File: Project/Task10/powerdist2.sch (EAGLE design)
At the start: 51 parts

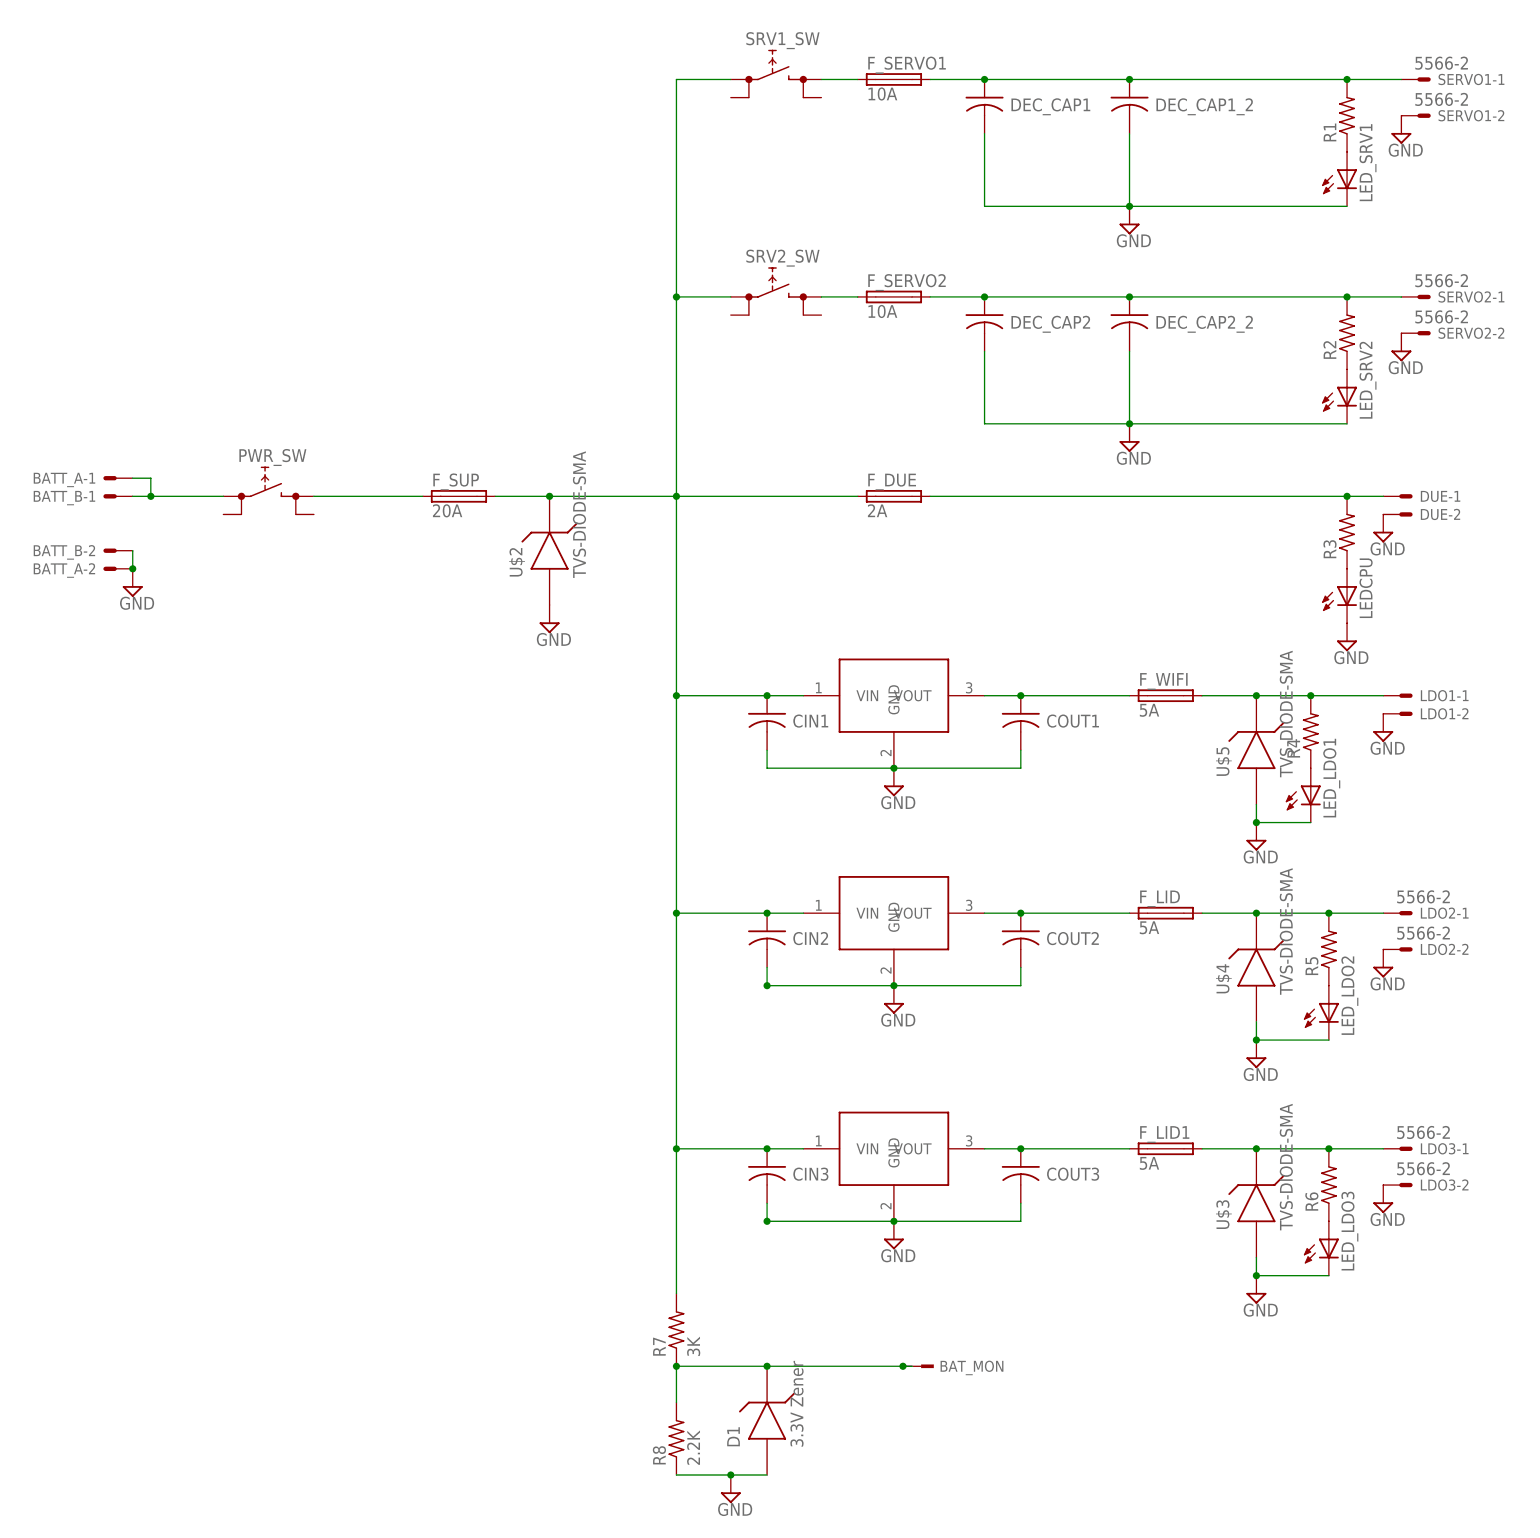
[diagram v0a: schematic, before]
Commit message: Updated Schematic, ready for submitting...
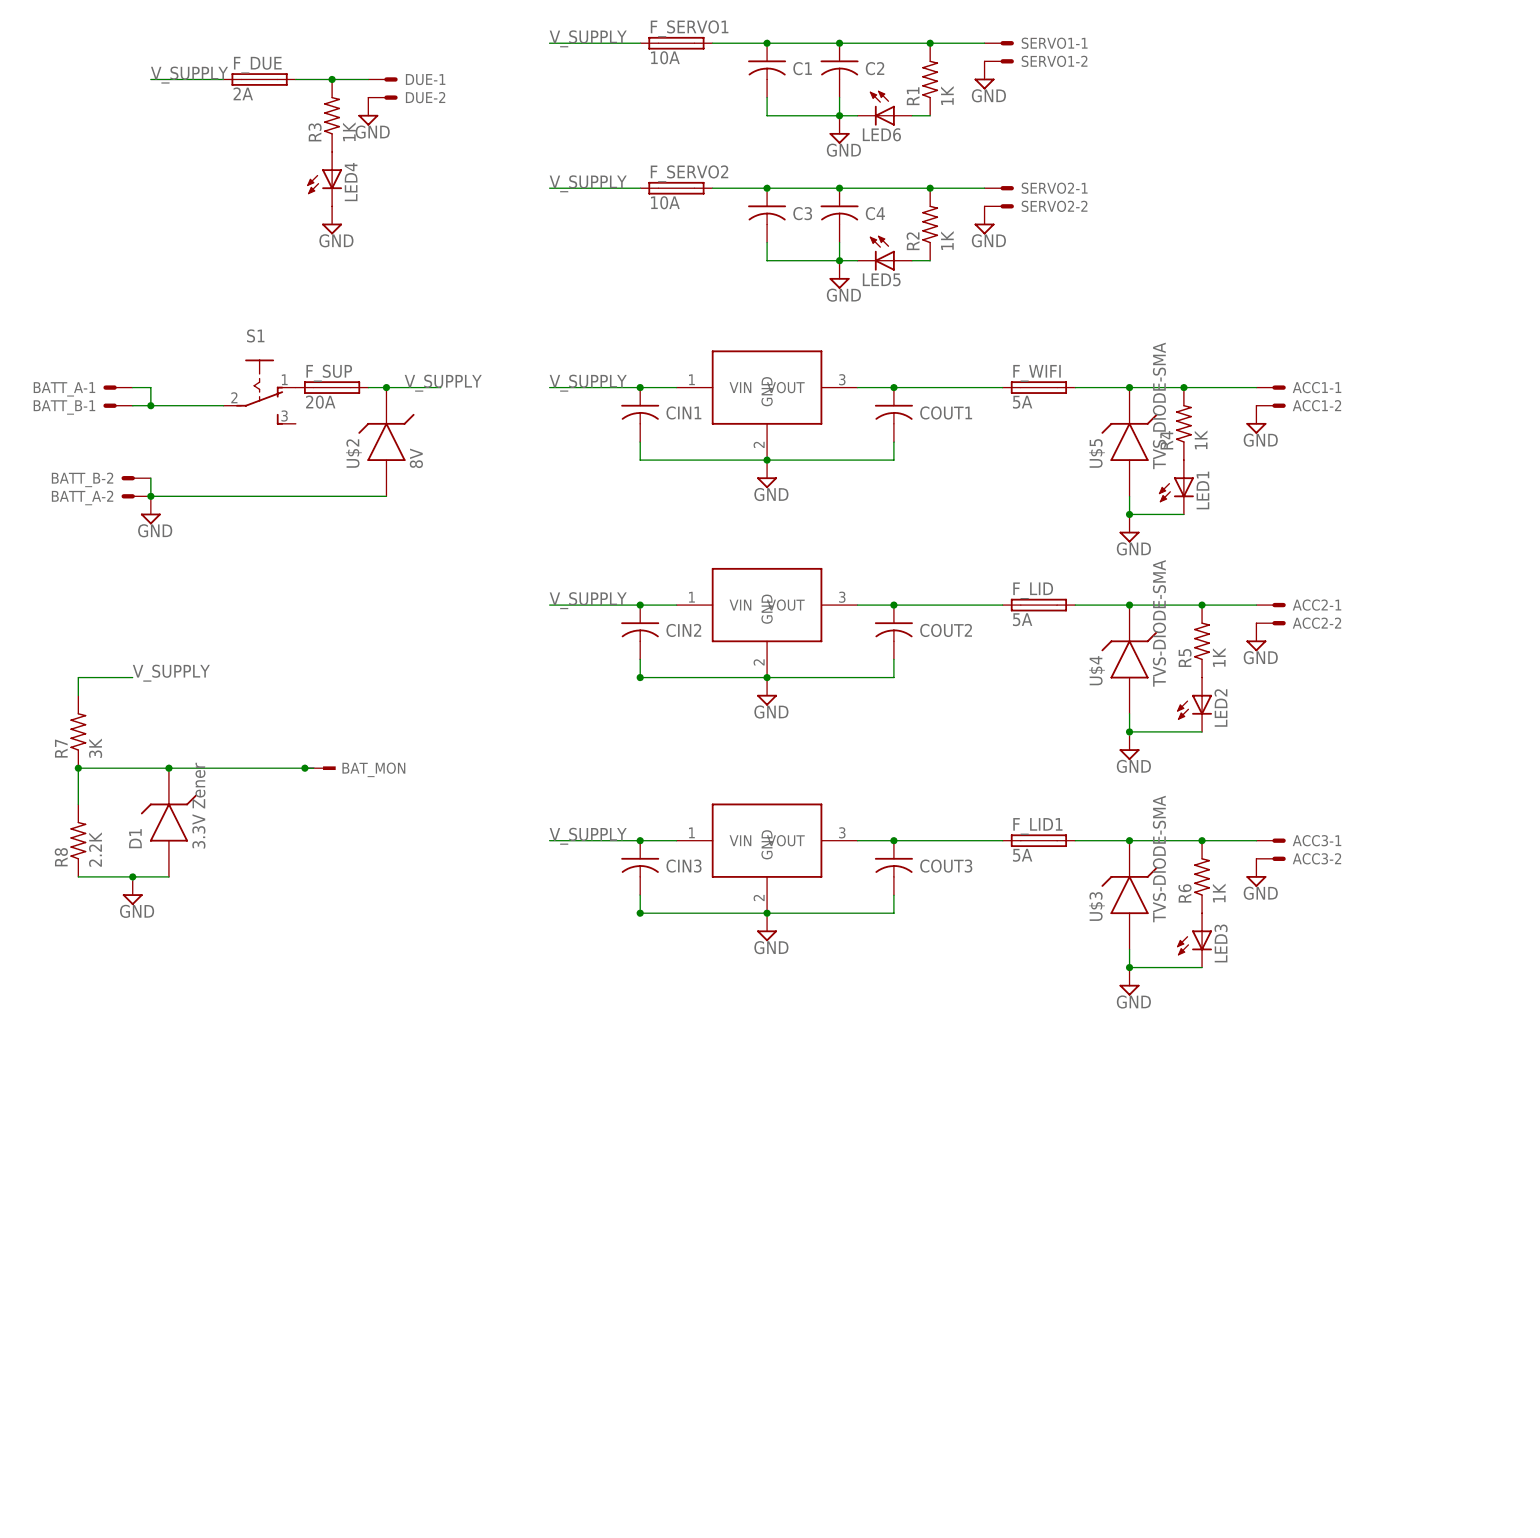
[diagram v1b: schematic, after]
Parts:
- removed DEC_CAP1, DEC_CAP1_2, DEC_CAP2, DEC_CAP2_2: CAPACITORTH_CAP, TinyGadget(1):CAPACITORTH_CAP
- removed LDO1: C-GRID-02-70553, con-molex:C-GRID-02-70553
- removed LDO2, LDO3: 5566-2, con-molex:5566-2
- removed LEDCPU, LED_LDO1, LED_LDO2, LED_LDO3, LED_SRV1, LED_SRV2: (no value), led:LEDCHIP-LED0805
- removed PWR_SW, SRV1_SW, SRV2_SW: (no value), switch:REKN
- added ACC1: C-GRID-02-70553, con-molex:C-GRID-02-70553
- added ACC2, ACC3: 5566-2, con-molex:5566-2
- added C1, C2, C3, C4: CAPACITORTH_CAP, TinyGadget(1):CAPACITORTH_CAP
- added LED1, LED2, LED3, LED4, LED5, LED6: (no value), led:LEDCHIP-LED0805
- added S1: (no value), switch:255SB
- R1, R2, R3, R4, R5, R6: value (none) -> 1K
- U$2: value TVS-DIODE-SMA -> 8V
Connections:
- removed net N$17: F_SERVO2.1, SRV2_SW.1@A
- removed net N$20: CIN1.1, CIN2.1, CIN3.1, F_DUE.1, F_SUP.2, R7.2, SRV1_SW.0@A, SRV2_SW.0@A, U$1.VIN, U$2.CAT, U$6.VIN, U$7.VIN
- removed net N$3: F_SERVO1.1, SRV1_SW.1@A
- new net V_SUPPLY: CIN1.1, CIN2.1, CIN3.1, F_DUE.1, F_SERVO1.1, F_SERVO2.1, F_SUP.2, R7.2, U$1.VIN, U$2.CAT, U$6.VIN, U$7.VIN
- net GND: now also ACC1-2.S, ACC2-2.S, ACC3-2.S, C1.2, C2.2, C3.2, C4.2, LED1.C, LED2.C, LED3.C, LED4.C, LED5.C, LED6.C; no longer DEC_CAP1.2, DEC_CAP1_2.2, DEC_CAP2.2, DEC_CAP2_2.2, LDO1-2.S, LDO2-2.S, LDO3-2.S, LEDCPU.C, LED_LDO1.C, LED_LDO2.C, LED_LDO3.C, LED_SRV1.C, LED_SRV2.C
- net N$1: now also C3.1, C4.1; no longer DEC_CAP2.1, DEC_CAP2_2.1
- net N$10: now also S1.P; no longer PWR_SW.0@A
- net N$11: now also LED4.A; no longer LEDCPU.A
- net N$13: now also LED1.A; no longer LED_LDO1.A
- net N$14: now also S1.O; no longer PWR_SW.1@A
- net N$15: now also C1.1, C2.1; no longer DEC_CAP1.1, DEC_CAP1_2.1
- net N$16: now also LED2.A; no longer LED_LDO2.A
- net N$2: now also ACC2-1.S; no longer LDO2-1.S
- net N$21: now also ACC3-1.S; no longer LDO3-1.S
- net N$22: now also LED3.A; no longer LED_LDO3.A
- net N$5: now also LED6.A; no longer LED_SRV1.A
- net N$7: now also ACC1-1.S; no longer LDO1-1.S
- net N$8: now also LED5.A; no longer LED_SRV2.A
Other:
- moved on the sheet: BATT_A-1, BATT_A-2, BATT_B-1, BATT_B-2, BAT_MON, CIN1, CIN2, CIN3, COUT1, COUT2, COUT3, D1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
